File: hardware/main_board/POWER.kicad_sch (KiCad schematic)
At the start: 7 parts, among them IC201 LM2937ET-3.3_NOPB, J201 373

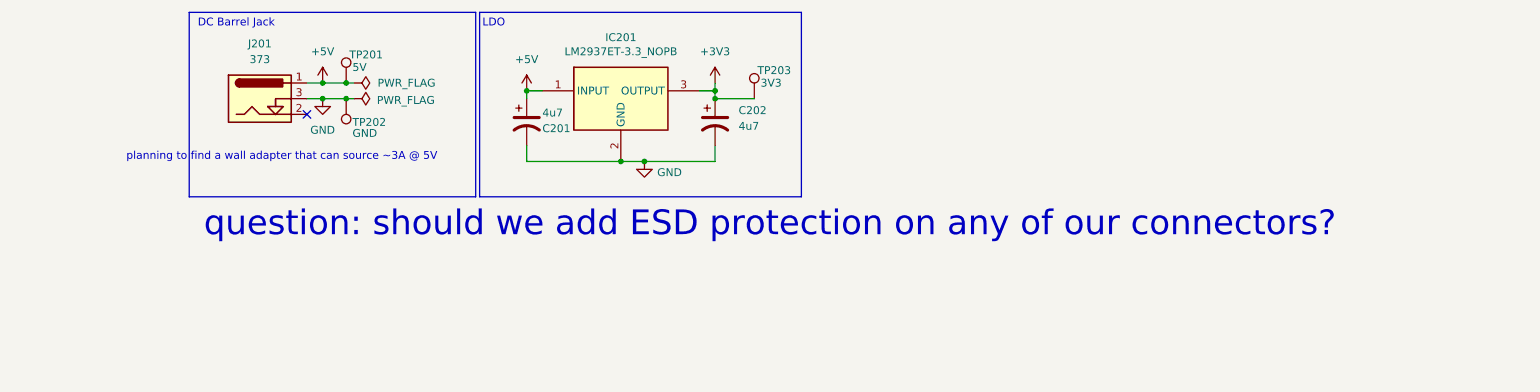
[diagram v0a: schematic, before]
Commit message: finished main pcb
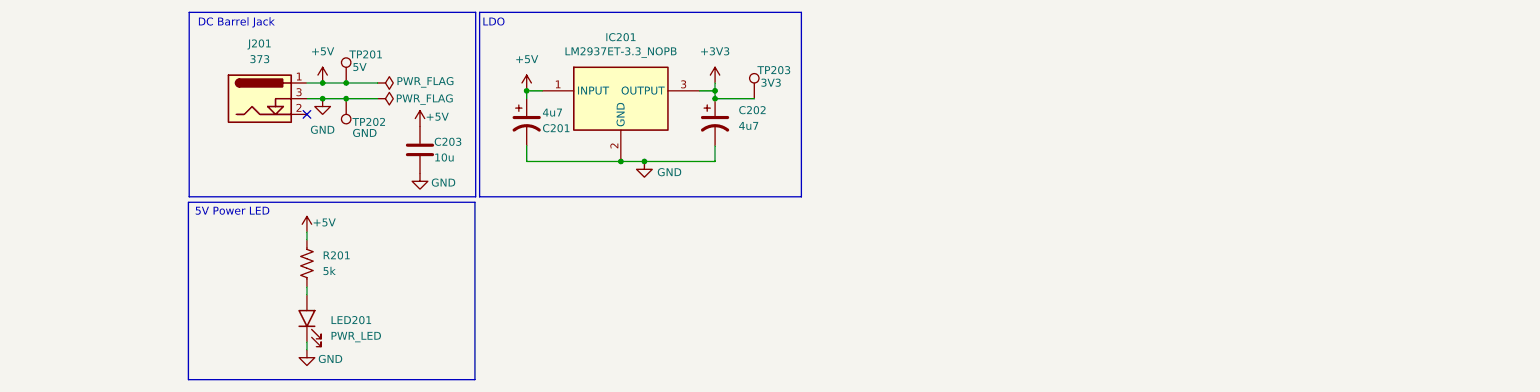
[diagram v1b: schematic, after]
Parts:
- added C203: 10u, Capacitor_SMD:C_0805_2012Metric, symbol ECE445L:C
- added LED201: PWR_LED, SamacSys_Parts:LEDC2012X40N, symbol ECE445L:LED
- added R201: 5k, Resistor_SMD:R_0805_2012Metric, symbol Device:R_US
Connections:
- net +5V: now also C203.1, R201.1
- net GND: now also C203.2, LED201.1 (K)
- new net: LED201.2 (A), R201.2
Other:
- note added: "5V Power LED"
- note removed: "planning to find a wall adapter that can source ~3A @ 5V"
- note removed: "question: should we add ESD protection on any of our connectors?"
